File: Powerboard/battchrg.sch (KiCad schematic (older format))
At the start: 48 parts, among them Q1(ACFET)? SI7617DN-T1-GE3

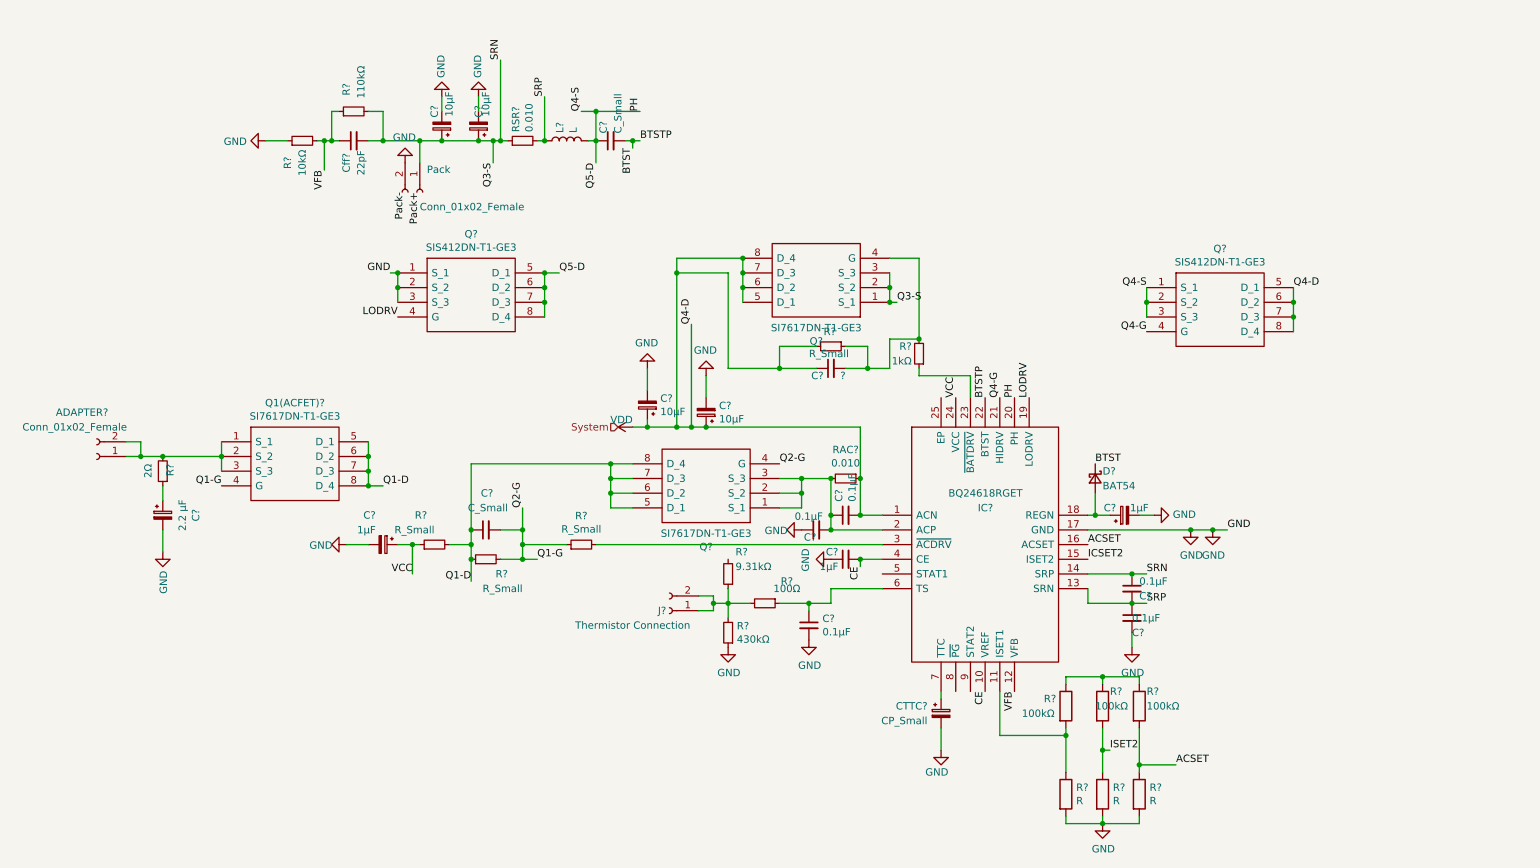
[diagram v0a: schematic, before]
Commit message: 01022022
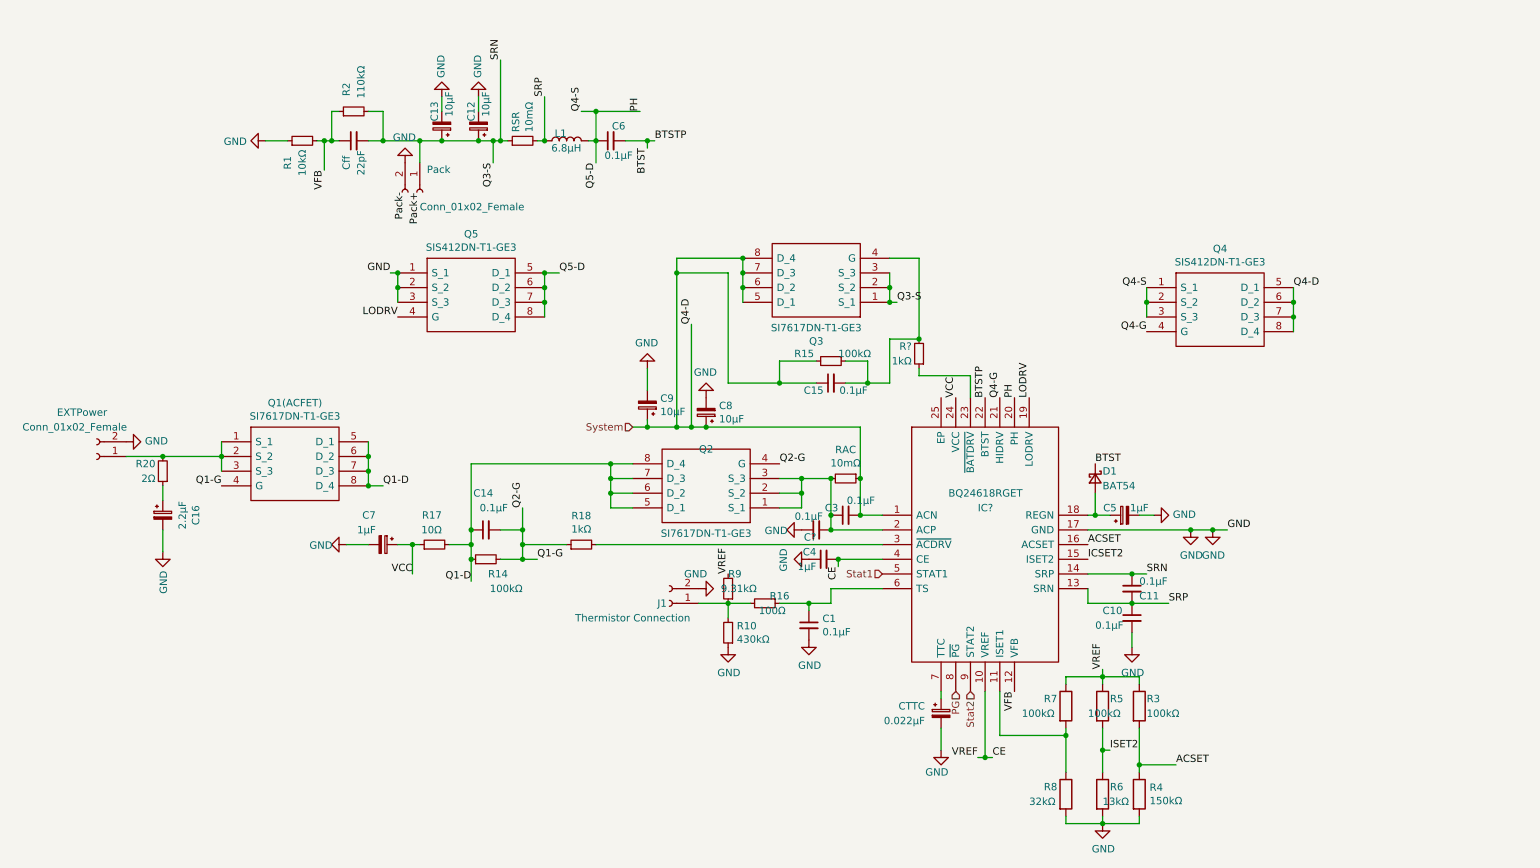
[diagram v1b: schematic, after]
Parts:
- C14, C6: renamed from C?; value C_Small -> 0.1µF
- C15: renamed from C?; value ? -> 0.1µF
- C16: renamed from C?; value 2.2 μF -> 2.2μF
- C7: renamed from C?; value 1μF -> 1µF
- CTTC: renamed from CTTC?; value CP_Small -> 0.022µF
- L1: renamed from L?; value L -> 6.8µH
- R14, R15: renamed from R?; value R_Small -> 100kΩ
- R17: renamed from R?; value R_Small -> 10Ω
- R18: renamed from R?; value R_Small -> 1kΩ
- R4: renamed from R?; value R -> 150kΩ
- R6: renamed from R?; value R -> 13kΩ
- R8: renamed from R?; value R -> 32kΩ
- RAC: renamed from RAC?; value 0.010 -> 10mΩ
- RSR: renamed from RSR?; value 0.010 -> 10mΩ
- gave numbers to parts that had none: 28
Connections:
- net VDD is gone; now on net System: C15.1, C3.2, C8.1, C9.1, IC?.1 (ACN), Q3.5 (D_1), Q3.6 (D_2), Q3.7 (D_3), Q3.8 (D_4), Q4.5 (D_1), Q4.6 (D_2), Q4.7 (D_3), Q4.8 (D_4), R15.2, RAC.1
- net CE: now also R3.1, R5.1, R7.1, R9.2
- net GND: now also EXTPower.2 (Pin_2), J1.2 (Pin_2)
- net at J1.1 (Pin_1), R10.2, R16.2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: no longer J1.2 (Pin_2)
- net Stat1: now reaches IC?.5 (STAT1)
- net PG: now reaches IC?.8 (~PG)
- net Stat2: now reaches IC?.9 (STAT2)
- net at EXTPower.1 (Pin_1), Q1(ACFET).1 (S_1), Q1(ACFET).2 (S_2)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: no longer EXTPower.2 (Pin_2)
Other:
- moved on the sheet: C15, C4, J1, R15, R9

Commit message: 08/02/2022 update3
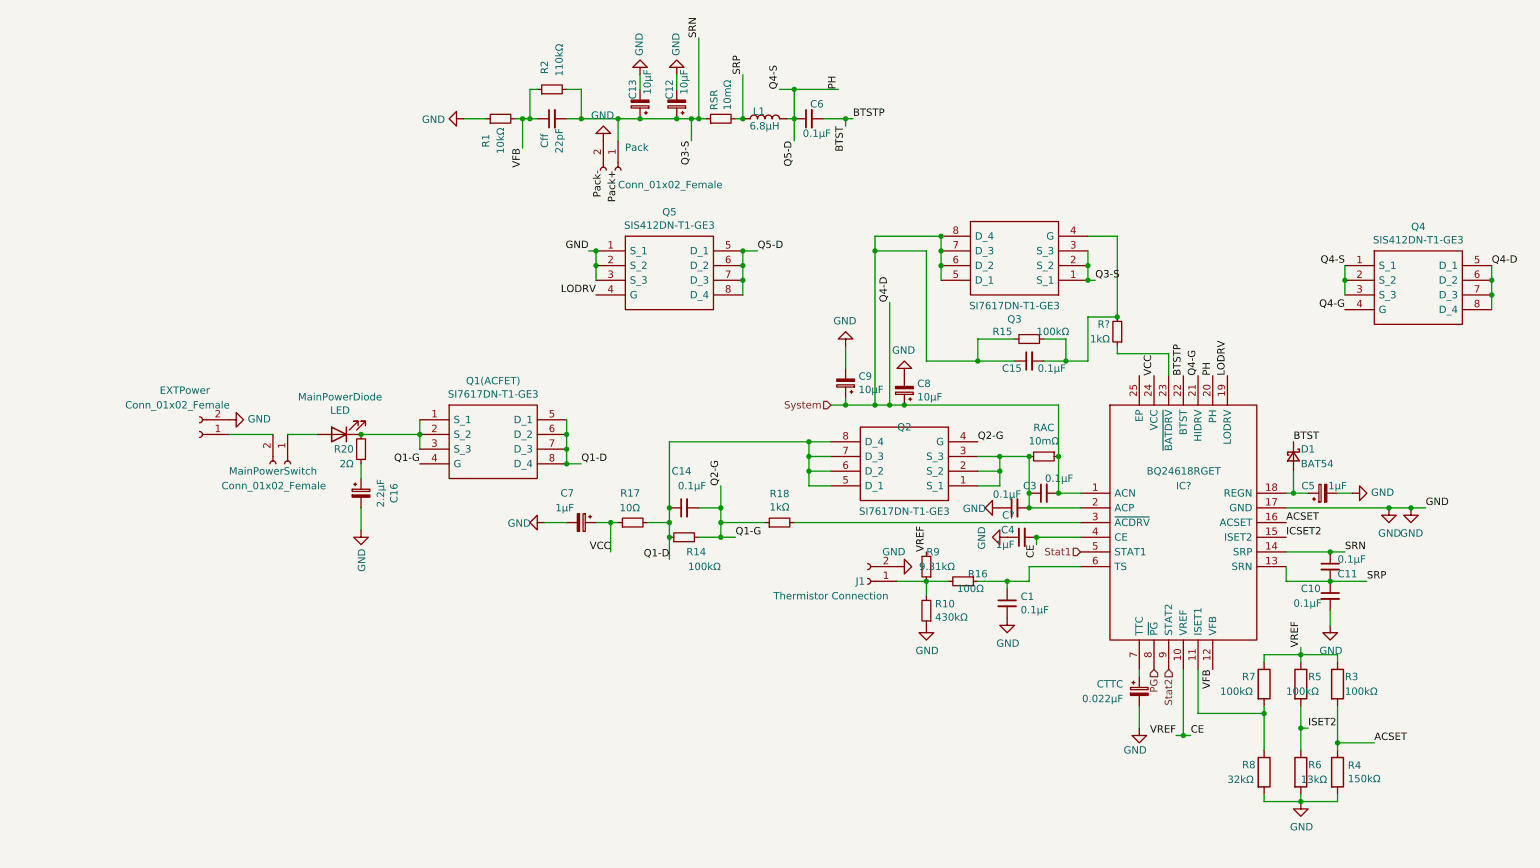
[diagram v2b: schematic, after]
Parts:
- added MainPowerDiode: LED, symbol Device:LED
- added MainPowerSwitch: Conn_01x02_Female, symbol Connector:Conn_01x02_Female
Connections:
- net at Q1(ACFET).1 (S_1), Q1(ACFET).2 (S_2), Q1(ACFET).3 (S_3)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: now also MainPowerDiode.1 (K); no longer EXTPower.1 (Pin_1)
- new net: EXTPower.1 (Pin_1), MainPowerSwitch.2 (Pin_2)
- new net: MainPowerDiode.2 (A), MainPowerSwitch.1 (Pin_1)
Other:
- moved on the sheet: C1, C10, C11, C12, C13, C14, C15, C16, C3, C4, C5, C6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
